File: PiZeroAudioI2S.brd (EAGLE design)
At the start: 65.3 x 30.3 mm, 69 parts, among them CON1 RPI-Header, J1 GROVE, J2 2X2HEADER, J3 2X1-LOCKING, J4 GROVE, J5 4X1-LOCKING, Q1 DMG2305UX, U1 TXB0104PWR, U2 LSM6DS33, U3 PCM5101A, U4 TXS0102, U5 TPA3144D2PWPR

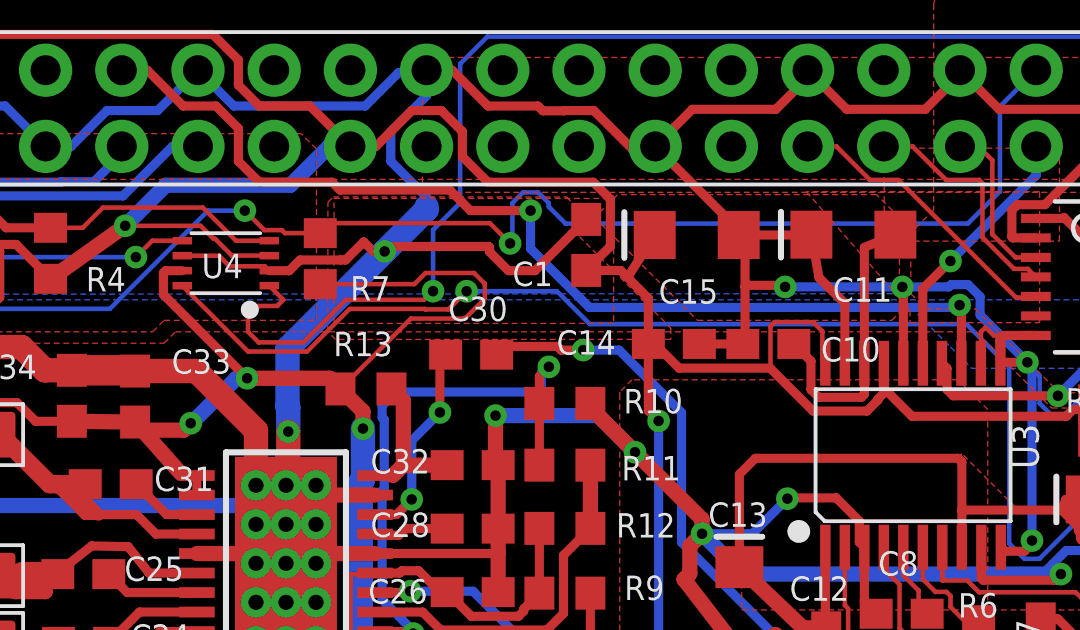
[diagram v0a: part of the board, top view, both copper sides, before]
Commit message: Update for Move account
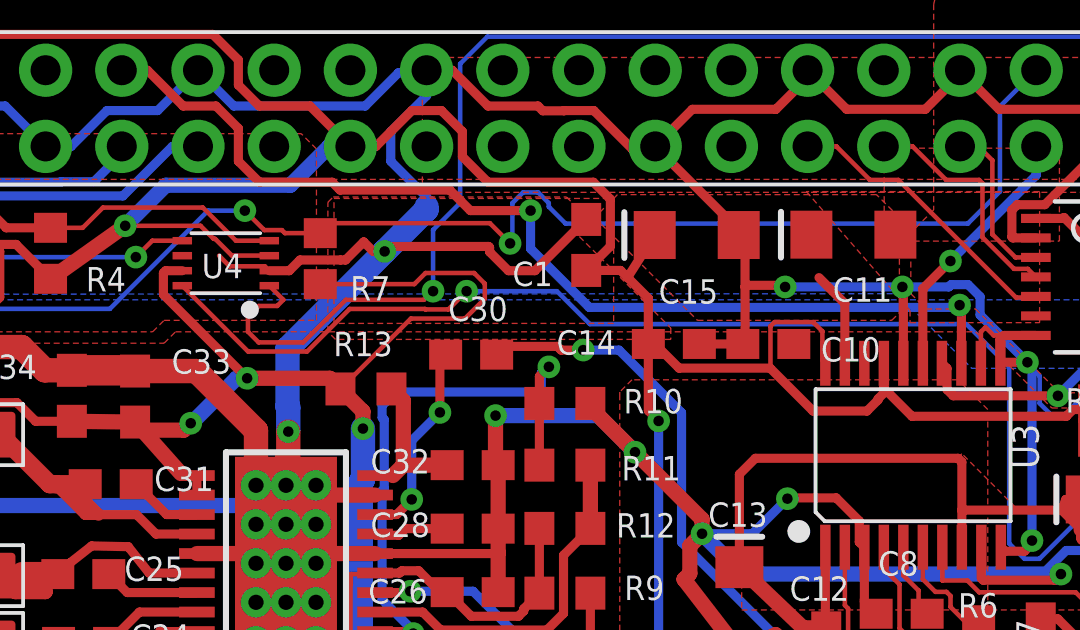
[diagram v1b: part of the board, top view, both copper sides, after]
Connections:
- net +3V3: now also U4.P$6
- net GND: now also C11.-; no longer C11.+, U4.P$6
- net N$12: now also C11.+; no longer C11.-
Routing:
- net N$12: track 9.70 -> 0.00 mm
- net GND: track 191.6 -> 186.2 mm
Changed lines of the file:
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@@
 <?xml version="1.0" encoding="utf-8"?>
 <!DOCTYPE eagle SYSTEM "eagle.dtd">
-<eagle version="9.1.3">
+<eagle version="9.4.1">
 <drawing>
 <settings>
@@
 <contactref element="C10" pad="2"/>
 <contactref element="C14" pad="1"/>
-<contactref element="C15" pad="-"/>
-<contactref element="C11" pad="+"/>
-<contactref element="U3" pad="19"/>
 <contactref element="U3" pad="10"/>
 <contactref element="U3" pad="11"/>
@@
 <wire x1="55.1434" y1="29.718" x2="55.1578" y2="29.7036" width="0.3048" layer="1"/>
 <wire x1="55.1578" y1="29.7036" x2="55.1578" y2="28.9222" width="0.3048" layer="1"/>
-<wire x1="46.6462" y1="33.276125" x2="46.4342" y2="33.1978" width="0.3048" layer="1"/>
 <wire x1="46.6462" y1="33.276125" x2="46.6462" y2="33.1564" width="0.3048" layer="1"/>
 <wire x1="46.6462" y1="29.64" x2="46.5718" y2="29.5656" width="0.3048" layer="1"/>
 <wire x1="46.5718" y1="29.5656" x2="45.1222" y2="29.5656" width="0.3048" layer="1"/>
-<wire x1="46.4342" y1="33.1978" x2="48.8452625" y2="33.1978" width="0.3048" layer="1"/>
-<wire x1="48.85669375" y1="33.20923125" x2="49.109609375" y2="31.779115625" width="0.3048" layer="1"/>
-<wire x1="49.109609375" y1="31.779115625" x2="49.9728" y2="30.915925" width="0.3048" layer="1"/>
-<wire x1="49.9728" y1="30.915925" x2="49.9728" y2="28.9222" width="0.3048" layer="1"/>
 <wire x1="55.1728" y1="22.7922" x2="55.3082" y2="22.6568" width="0.3048" layer="1"/>
 <wire x1="55.3082" y1="22.6568" x2="55.9562" y2="22.6568" width="0.3048" layer="1"/>
@@
 <wire x1="46.6462" y1="33.1564" x2="46.6462" y2="31.4706" width="0.3048" layer="1"/>
 <wire x1="46.6462" y1="31.4706" x2="46.6462" y2="29.64" width="0.3048" layer="1"/>
-<wire x1="48.8452625" y1="33.1978" x2="48.85669375" y2="33.20923125" width="0.3048" layer="1"/>
 <wire x1="46.6462" y1="31.4706" x2="46.697" y2="31.5214" width="0.3048" layer="1"/>
 <wire x1="47.927003125" y1="31.5214" x2="47.9806" y2="31.467803125" width="0.3048" layer="1"/>
@@
 <wire x1="54.6608" y1="30.1244" x2="54.9344" y2="29.8508" width="0.1524" layer="1"/>
 <wire x1="54.9344" y1="29.8508" x2="55.2762" y2="29.8508" width="0.1524" layer="1"/>
-<contactref element="U4" pad="P$6"/>
 <wire x1="30.6406" y1="32.1544" x2="30.787" y2="32.008" width="0.1524" layer="1"/>
 <wire x1="29.46674375" y1="32.1544" x2="29.11314375" y2="32.508" width="0.1524" layer="1"/>
@@
 <wire x1="56.467" y1="27.58705" x2="56.467" y2="28.496" width="0.1524" layer="16"/>
 <wire x1="56.467" y1="28.496" x2="56.0578" y2="28.9052" width="0.1524" layer="16"/>
-<wire x1="29.11314375" y1="32.508" x2="27.887" y2="32.508" width="0.1524" layer="1"/>
 <wire x1="10.8966" y1="34.4424" x2="10.834" y2="34.4424" width="0.3048" layer="1"/>
 <wire x1="38.131" y1="32.6354875" x2="38.131" y2="32.7858" width="0.3048" layer="1"/>
@@
 <wire x1="34.798" y1="32.8168" x2="34.6329" y2="32.6517" width="0.3048" layer="1"/>
 <wire x1="12.66850625" y1="39.8782" x2="17.0644" y2="39.8782" width="0.254" layer="16"/>
+<contactref element="C11" pad="-"/>
+<contactref element="U3" pad="19"/>
+<wire x1="49.109609375" y1="31.779115625" x2="49.9728" y2="30.915925" width="0.3048" layer="1"/>
+<wire x1="49.9728" y1="30.915925" x2="49.9728" y2="28.9222" width="0.3048" layer="1"/>
+<contactref element="C15" pad="-"/>
+<wire x1="51.8898" y1="31.4678" x2="51.65669375" y2="33.20923125" width="0" layer="19" extent="1-1"/>
+<wire x1="46.4342" y1="33.1978" x2="46.6462" y2="33.276125" width="0" layer="19" extent="1-1"/>
+<wire x1="49.109609375" y1="31.779115625" x2="47.9806" y2="31.467803125" width="0" layer="19" extent="1-16"/>
 </signal>
 <signal name="PCM_FS">
@@
 <wire x1="39.8526" y1="12.7762" x2="39.8526" y2="13.804" width="0.3048" layer="1"/>
 <wire x1="39.8526" y1="13.804" x2="38.3912" y2="15.2654" width="0.3048" layer="1"/>
+<contactref element="U4" pad="P$6"/>
+<wire x1="28.496" y1="33.5054" x2="27.887" y2="32.508" width="0" layer="19" extent="1-1"/>
 </signal>
 <signal name="SDA">
@@
 <wire x1="50.0808" y1="18.7532" x2="50.3428" y2="18.4912" width="0.1524" layer="1"/>
 </signal>
-<signal name="N$12">
-<contactref element="U3" pad="18"/>
-<contactref element="C11" pad="-"/>
-<contactref element="C10" pad="1"/>
-<wire x1="50.6228" y1="28.9222" x2="50.6228" y2="32.785271875" width="0.3048" layer="1"/>
-<wire x1="50.6228" y1="32.785271875" x2="51.65669375" y2="33.20923125" width="0.3048" layer="1"/>
-<wire x1="48.2718" y1="29.5656" x2="48.843" y2="28.9944" width="0.3048" layer="1"/>
-<wire x1="48.843" y1="28.9944" x2="48.843" y2="28.04595" width="0.3048" layer="1"/>
-<wire x1="48.843" y1="28.04595" x2="49.10135" y2="27.7876" width="0.3048" layer="1"/>
-<wire x1="49.10135" y1="27.7876" x2="50.5206" y2="27.7876" width="0.3048" layer="1"/>
-<wire x1="50.5206" y1="27.7876" x2="50.6228" y2="27.8898" width="0.3048" layer="1"/>
-<wire x1="50.6228" y1="27.8898" x2="50.6228" y2="28.9222" width="0.3048" layer="1"/>
-</signal>
 <signal name="N$11">
 <contactref element="U3" pad="6"/>
@@
 <wire x1="35.0306" y1="23.88" x2="34.3136" y2="23.88" width="0.3048" layer="1"/>
 </signal>
+<signal name="N$12">
+<contactref element="U3" pad="18"/>
+<contactref element="C11" pad="+"/>
+<contactref element="C10" pad="1"/>
+<wire x1="48.2718" y1="29.5656" x2="48.85669375" y2="33.20923125" width="0" layer="19" extent="1-1"/>
+<wire x1="50.6228" y1="28.9222" x2="48.2718" y2="29.5656" width="0" layer="19" extent="1-1"/>
+</signal>
 </signals>
